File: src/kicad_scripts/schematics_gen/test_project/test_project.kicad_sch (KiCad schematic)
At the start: 2 parts

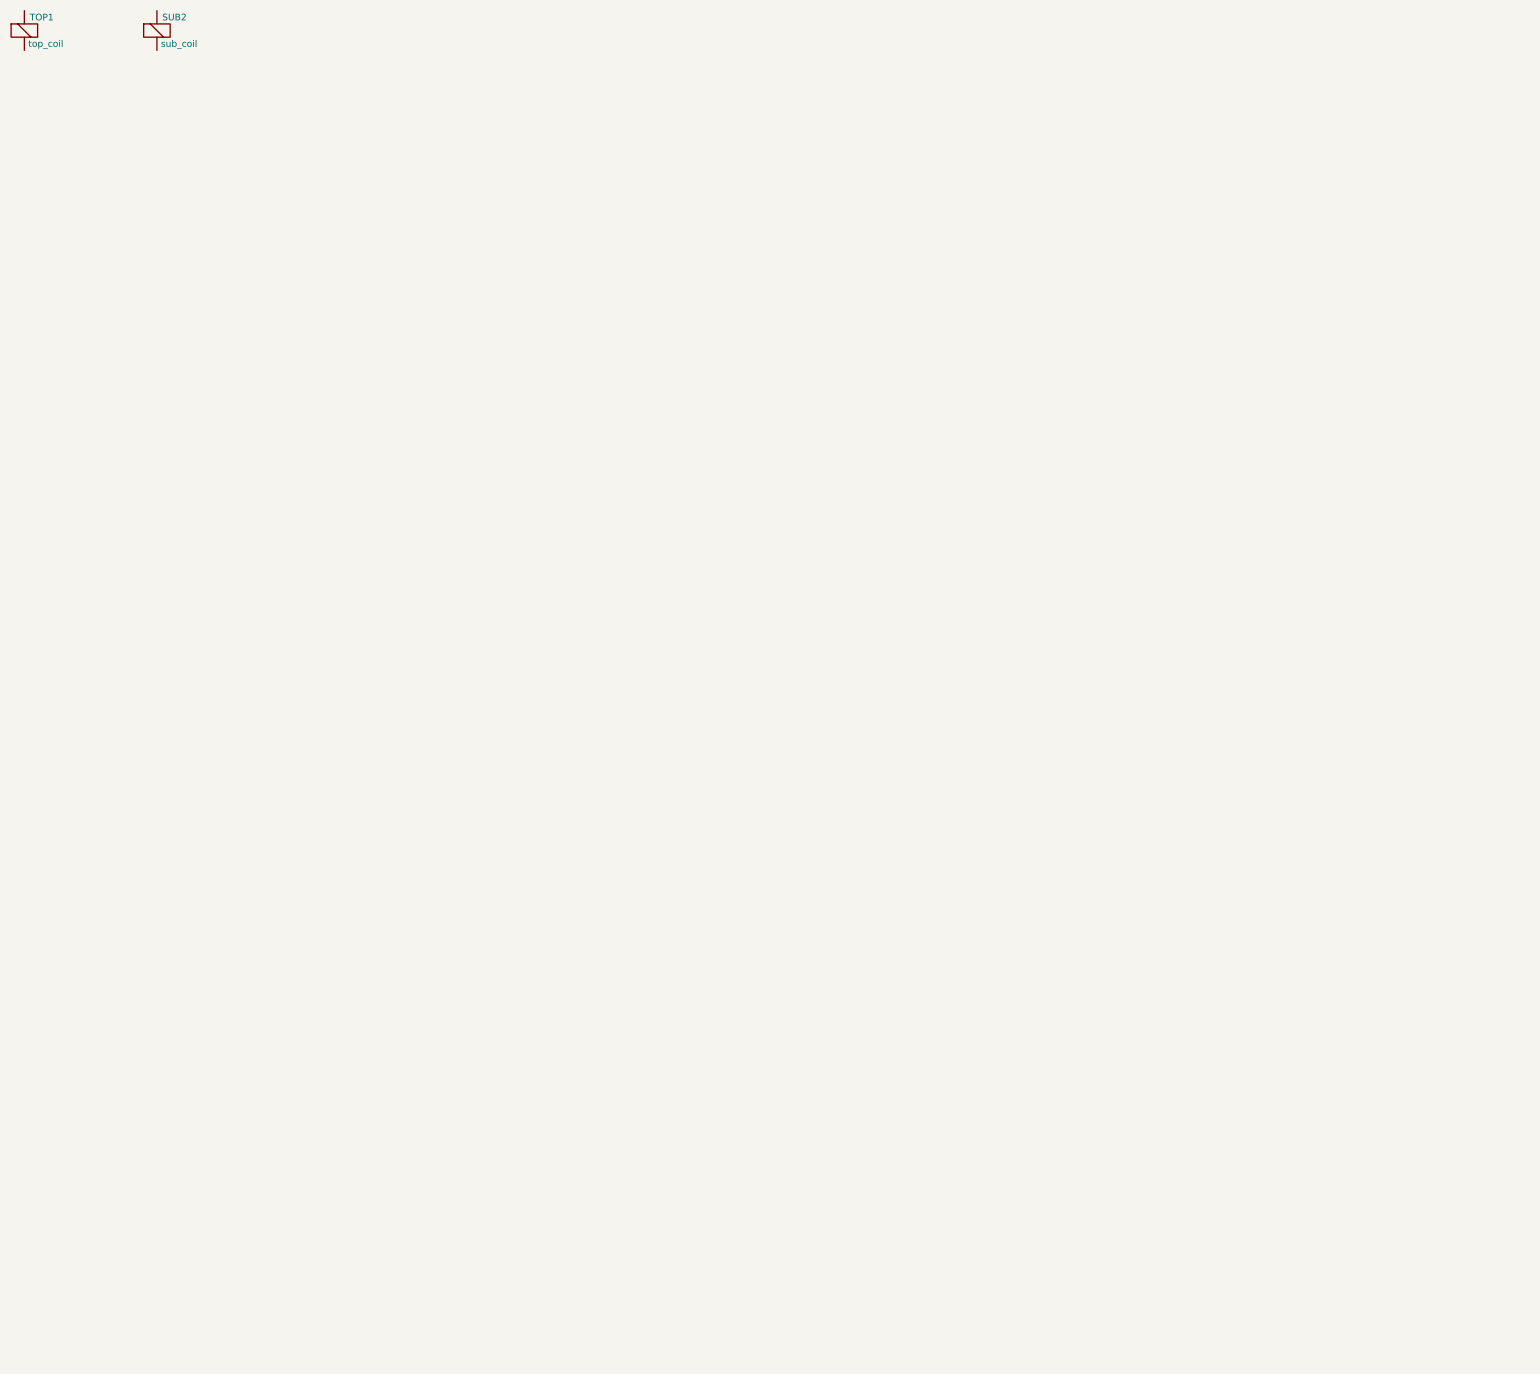
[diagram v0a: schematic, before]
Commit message: Before turning components in schematics maker
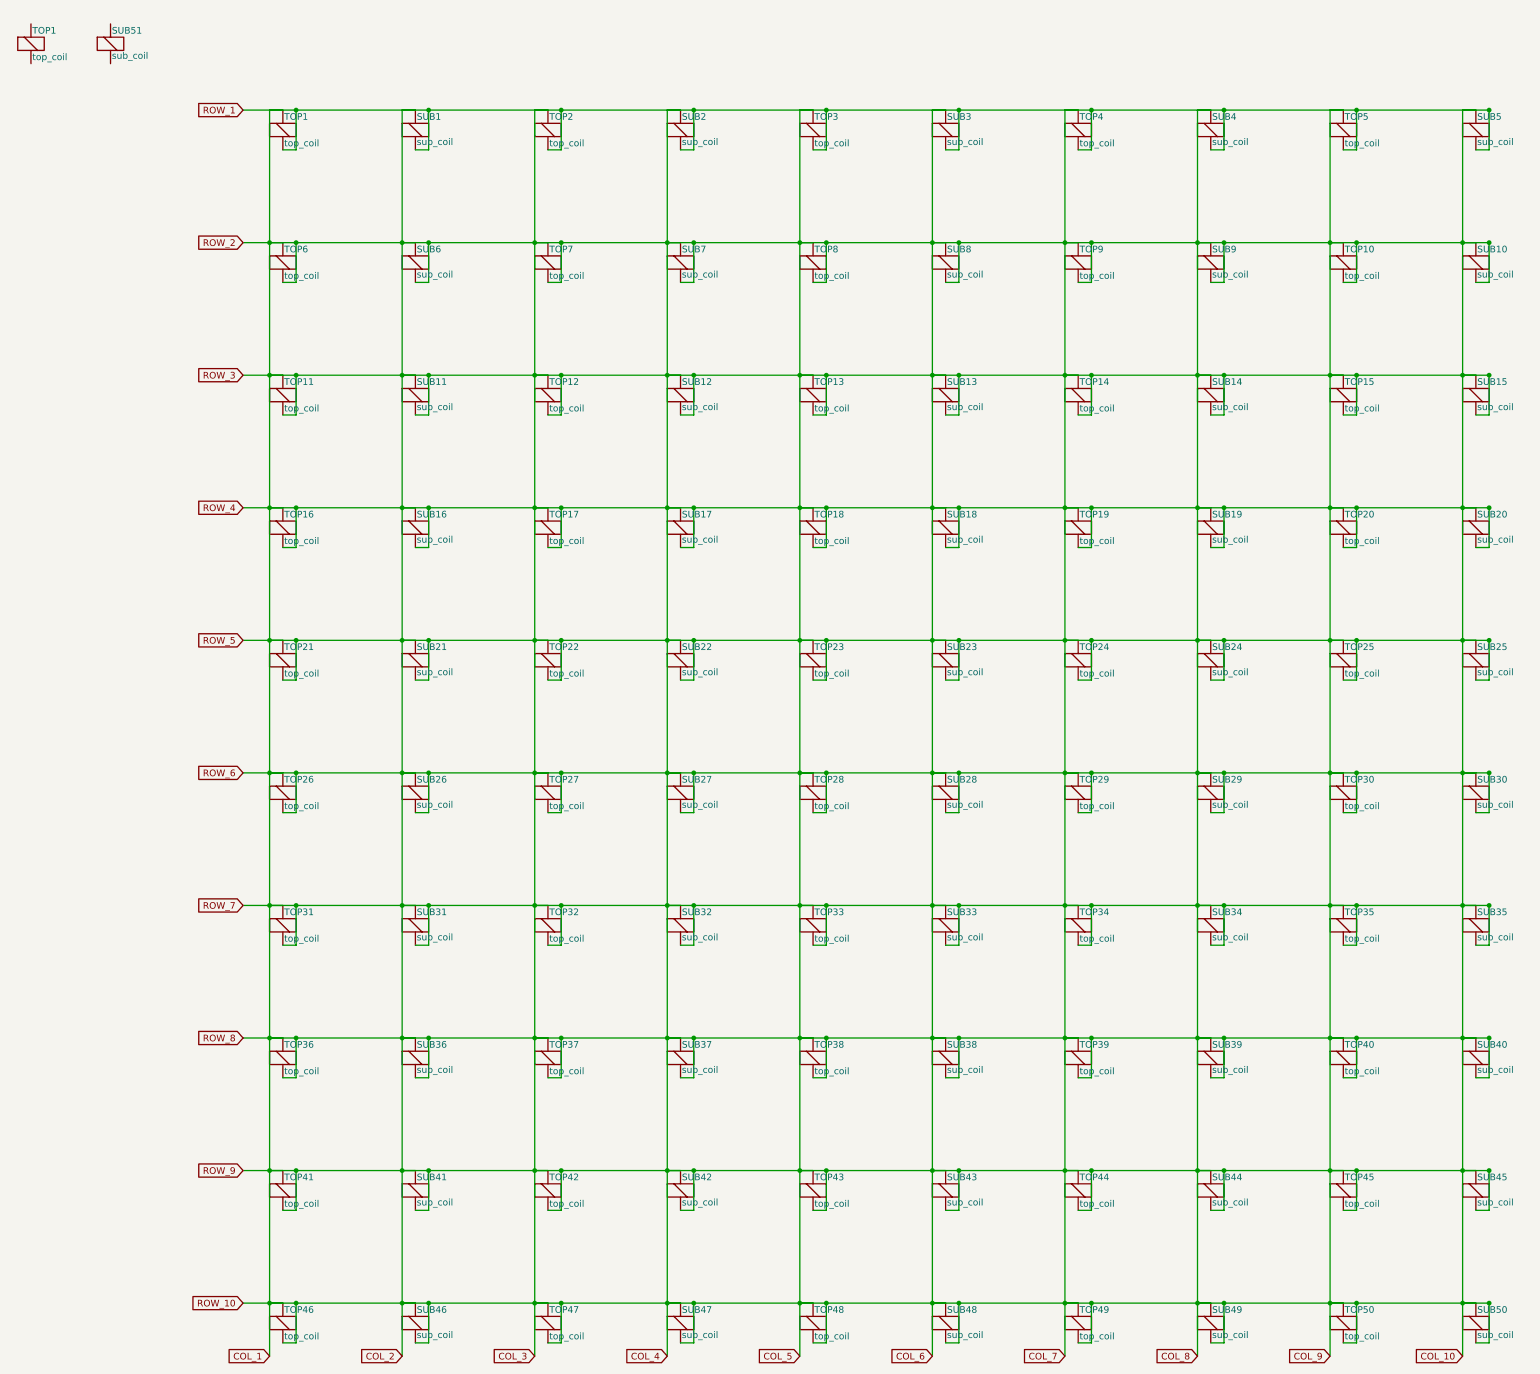
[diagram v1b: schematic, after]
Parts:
- removed SUB2: sub_coil, sub_coils:sub_coil, symbol Device:ElectromagneticActor
- removed TOP1: top_coil, sub_coils:top_coil, symbol Device:ElectromagneticActor
- added SUB1, SUB10, SUB11, SUB12, SUB13, SUB14, SUB15, SUB16, SUB17, SUB18, SUB19, SUB2, SUB20, SUB21, SUB22, SUB23, SUB24, SUB25, SUB26, SUB27, SUB28, SUB29, SUB3, SUB30, SUB31, SUB32, SUB33, SUB34, SUB35, SUB36, SUB37, SUB38, SUB39, SUB4, SUB40, SUB41, SUB42, SUB43, SUB44, SUB45, SUB46, SUB47, SUB48, SUB49, SUB5, SUB50, SUB51, SUB6, SUB7, SUB8, SUB9: sub_coil, sub_coils:top_coil, symbol square_coils:sub_coil
- added TOP1 (x2), TOP10, TOP11, TOP12, TOP13, TOP14, TOP15, TOP16, TOP17, TOP18, TOP19, TOP2, TOP20, TOP21, TOP22, TOP23, TOP24, TOP25, TOP26, TOP27, TOP28, TOP29, TOP3, TOP30, TOP31, TOP32, TOP33, TOP34, TOP35, TOP36, TOP37, TOP38, TOP39, TOP4, TOP40, TOP41, TOP42, TOP43, TOP44, TOP45, TOP46, TOP47, TOP48, TOP49, TOP5, TOP50, TOP6, TOP7, TOP8, TOP9: top_coil, sub_coils:top_coil, symbol square_coils:top_coil
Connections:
- new net COL_1: SUB1.1 (A), SUB1.2 (B), SUB10.1 (A), SUB10.2 (B), SUB11.1 (A), SUB11.2 (B), SUB12.1 (A), SUB12.2 (B), SUB13.1 (A), SUB13.2 (B), SUB14.1 (A), SUB14.2 (B), SUB15.1 (A), SUB15.2 (B), SUB16.1 (A), SUB16.2 (B), SUB17.1 (A), SUB17.2 (B), SUB18.1 (A), SUB18.2 (B), SUB19.1 (A), SUB19.2 (B), SUB2.1 (A), SUB2.2 (B), SUB20.1 (A), SUB20.2 (B), SUB21.1 (A), SUB21.2 (B), SUB22.1 (A), SUB22.2 (B), SUB23.1 (A), SUB23.2 (B), SUB24.1 (A), SUB24.2 (B), SUB25.1 (A), SUB25.2 (B), SUB26.1 (A), SUB26.2 (B), SUB27.1 (A), SUB27.2 (B), SUB28.1 (A), SUB28.2 (B), SUB29.1 (A), SUB29.2 (B), SUB3.1 (A), SUB3.2 (B), SUB30.1 (A), SUB30.2 (B), SUB31.1 (A), SUB31.2 (B), SUB32.1 (A), SUB32.2 (B), SUB33.1 (A), SUB33.2 (B), SUB34.1 (A), SUB34.2 (B), SUB35.1 (A), SUB35.2 (B), SUB36.1 (A), SUB36.2 (B), SUB37.1 (A), SUB37.2 (B), SUB38.1 (A), SUB38.2 (B), SUB39.1 (A), SUB39.2 (B), SUB4.1 (A), SUB4.2 (B), SUB40.1 (A), SUB40.2 (B), SUB41.1 (A), SUB41.2 (B), SUB42.1 (A), SUB42.2 (B), SUB43.1 (A), SUB43.2 (B), SUB44.1 (A), SUB44.2 (B), SUB45.1 (A), SUB45.2 (B), SUB46.1 (A), SUB46.2 (B), SUB47.1 (A), SUB47.2 (B), SUB48.1 (A), SUB48.2 (B), SUB49.1 (A), SUB49.2 (B), SUB5.1 (A), SUB5.2 (B), SUB50.1 (A), SUB50.2 (B), SUB6.1 (A), SUB6.2 (B), SUB7.1 (A), SUB7.2 (B), SUB8.1 (A), SUB8.2 (B), SUB9.1 (A), SUB9.2 (B), TOP1.1 (A), TOP1.2 (B), TOP10.1 (A), TOP10.2 (B), TOP11.1 (A), TOP11.2 (B), TOP12.1 (A), TOP12.2 (B), TOP13.1 (A), TOP13.2 (B), TOP14.1 (A), TOP14.2 (B), TOP15.1 (A), TOP15.2 (B), TOP16.1 (A), TOP16.2 (B), TOP17.1 (A), TOP17.2 (B), TOP18.1 (A), TOP18.2 (B), TOP19.1 (A), TOP19.2 (B), TOP2.1 (A), TOP2.2 (B), TOP20.1 (A), TOP20.2 (B), TOP21.1 (A), TOP21.2 (B), TOP22.1 (A), TOP22.2 (B), TOP23.1 (A), TOP23.2 (B), TOP24.1 (A), TOP24.2 (B), TOP25.1 (A), TOP25.2 (B), TOP26.1 (A), TOP26.2 (B), TOP27.1 (A), TOP27.2 (B), TOP28.1 (A), TOP28.2 (B), TOP29.1 (A), TOP29.2 (B), TOP3.1 (A), TOP3.2 (B), TOP30.1 (A), TOP30.2 (B), TOP31.1 (A), TOP31.2 (B), TOP32.1 (A), TOP32.2 (B), TOP33.1 (A), TOP33.2 (B), TOP34.1 (A), TOP34.2 (B), TOP35.1 (A), TOP35.2 (B), TOP36.1 (A), TOP36.2 (B), TOP37.1 (A), TOP37.2 (B), TOP38.1 (A), TOP38.2 (B), TOP39.1 (A), TOP39.2 (B), TOP4.1 (A), TOP4.2 (B), TOP40.1 (A), TOP40.2 (B), TOP41.1 (A), TOP41.2 (B), TOP42.1 (A), TOP42.2 (B), TOP43.1 (A), TOP43.2 (B), TOP44.1 (A), TOP44.2 (B), TOP45.1 (A), TOP45.2 (B), TOP46.1 (A), TOP46.2 (B), TOP47.1 (A), TOP47.2 (B), TOP48.1 (A), TOP48.2 (B), TOP49.1 (A), TOP49.2 (B), TOP5.1 (A), TOP5.2 (B), TOP50.1 (A), TOP50.2 (B), TOP6.1 (A), TOP6.2 (B), TOP7.1 (A), TOP7.2 (B), TOP8.1 (A), TOP8.2 (B), TOP9.1 (A), TOP9.2 (B)
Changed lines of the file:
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@@
-(kicad_sch
-	(version 20231120)
-	(generator "eeschema")
-	(generator_version "8.0")
-	(paper "A3")
-	(symbol
-		(lib_id "Device:ElectromagneticActor")
-		(at -25.4 -17.78 0)
-		(unit 1)
-		(exclude_from_sim no)
-		(in_bom yes)
-		(on_board yes)
-		(dnp no)
-		(property "Reference" "SUB2"
-			(at -24.384 -21.59 0)
-			(effects
-				(font
-					(size 1.27 1.27)
-				)
-				(justify left)
-			)
-		)
-		(property "Value" "sub_coil"
-			(at -24.638 -16.51 0)
-			(effects
-				(font
-					(size 1.27 1.27)
-				)
-				(justify left)
-			)
-		)
-		(property "Footprint" "sub_coils:sub_coil"
-			(at -26.035 -20.32 90)
-			(effects
-				(font
-					(size 1.27 1.27)
-				)
-				(hide yes)
-			)
-		)
-		(property "Datasheet" "~"
-			(at -26.035 -20.32 90)
-			(effects
-				(font
-					(size 1.27 1.27)
-				)
-				(hide yes)
-			)
-		)
-		(property "Description" "Electromagnetic actor"
-			(at -25.4 -17.78 0)
-			(effects
-				(font
-					(size 1.27 1.27)
-				)
-				(hide yes)
-			)
-		)
-		(pin "2"
-		)
-		(pin "1"
-		)
-		(instances
-			(project "test_project"
-				(path "/11af7b42-8094-4ca6-9444-8e07a1921bec"
-					(reference "SUB2")
-					(unit 1)
-				)
-			)
-		)
-	)
-	(symbol
-		(lib_id "Device:ElectromagneticActor")
-		(at -50.8 -17.78 0)
-		(unit 1)
-		(exclude_from_sim no)
-		(in_bom yes)
-		(on_board yes)
-		(dnp no)
-		(property "Reference" "TOP1"
-			(at -49.784 -21.59 0)
-			(effects
-				(font
-					(size 1.27 1.27)
-				)
-				(justify left)
-			)
-		)
-		(property "Value" "top_coil"
-			(at -50.038 -16.51 0)
-			(effects
-				(font
-					(size 1.27 1.27)
-				)
-				(justify left)
-			)
-		)
-		(property "Footprint" "sub_coils:top_coil"
-			(at -51.435 -20.32 90)
-			(effects
-				(font
-					(size 1.27 1.27)
-				)
-				(hide yes)
-			)
-		)
-		(property "Datasheet" "~"
-			(at -51.435 -20.32 90)
-			(effects
-				(font
-					(size 1.27 1.27)
-				)
-				(hide yes)
-			)
-		)
-		(property "Description" "Electromagnetic actor"
-			(at -50.8 -17.78 0)
-			(effects
-				(font
-					(size 1.27 1.27)
-				)
-				(hide yes)
-			)
-		)
-		(pin "2"
-		)
-		(pin "1"
-		)
-		(instances
-			(project "test_project"
-				(path "/11af7b42-8094-4ca6-9444-8e07a1921bec"
-					(reference "TOP1")
-					(unit 1)
-				)
-			)
-		)
-	)
-	(sheet_instances
-		(path "/"
-			(page "1")
-		)
-	)
-)
